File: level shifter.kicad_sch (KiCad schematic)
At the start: 81 parts, among them U501 TL074, U801 TL074

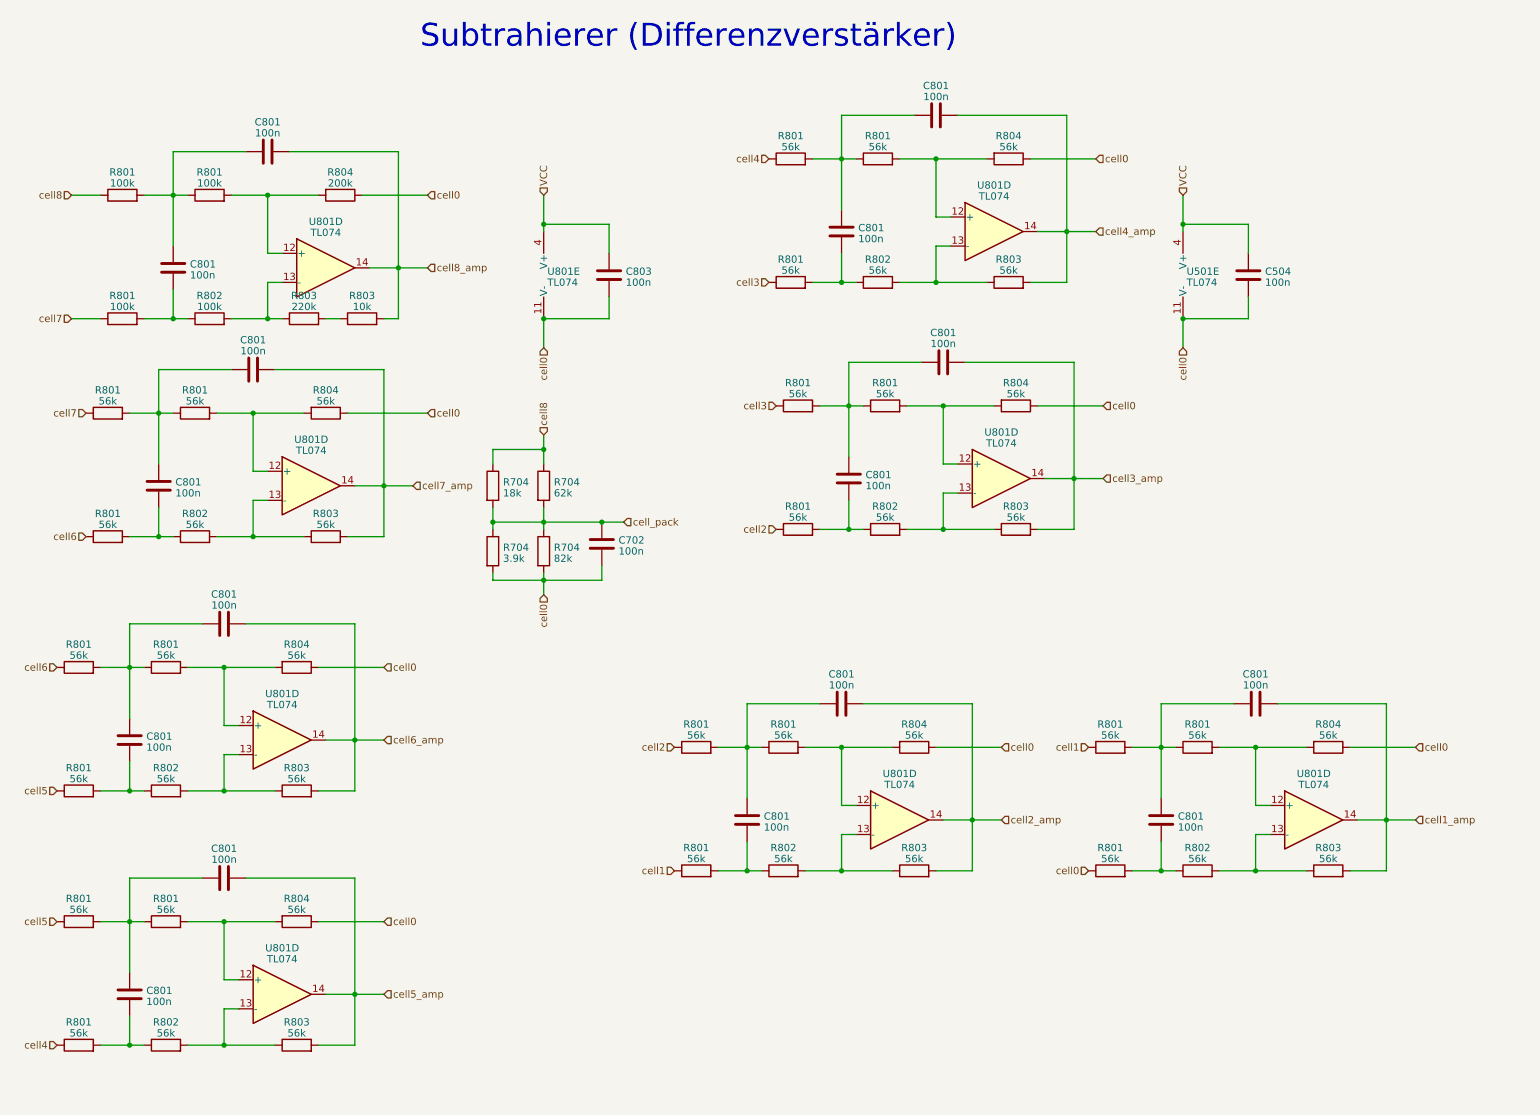
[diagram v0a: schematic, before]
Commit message: githubstart
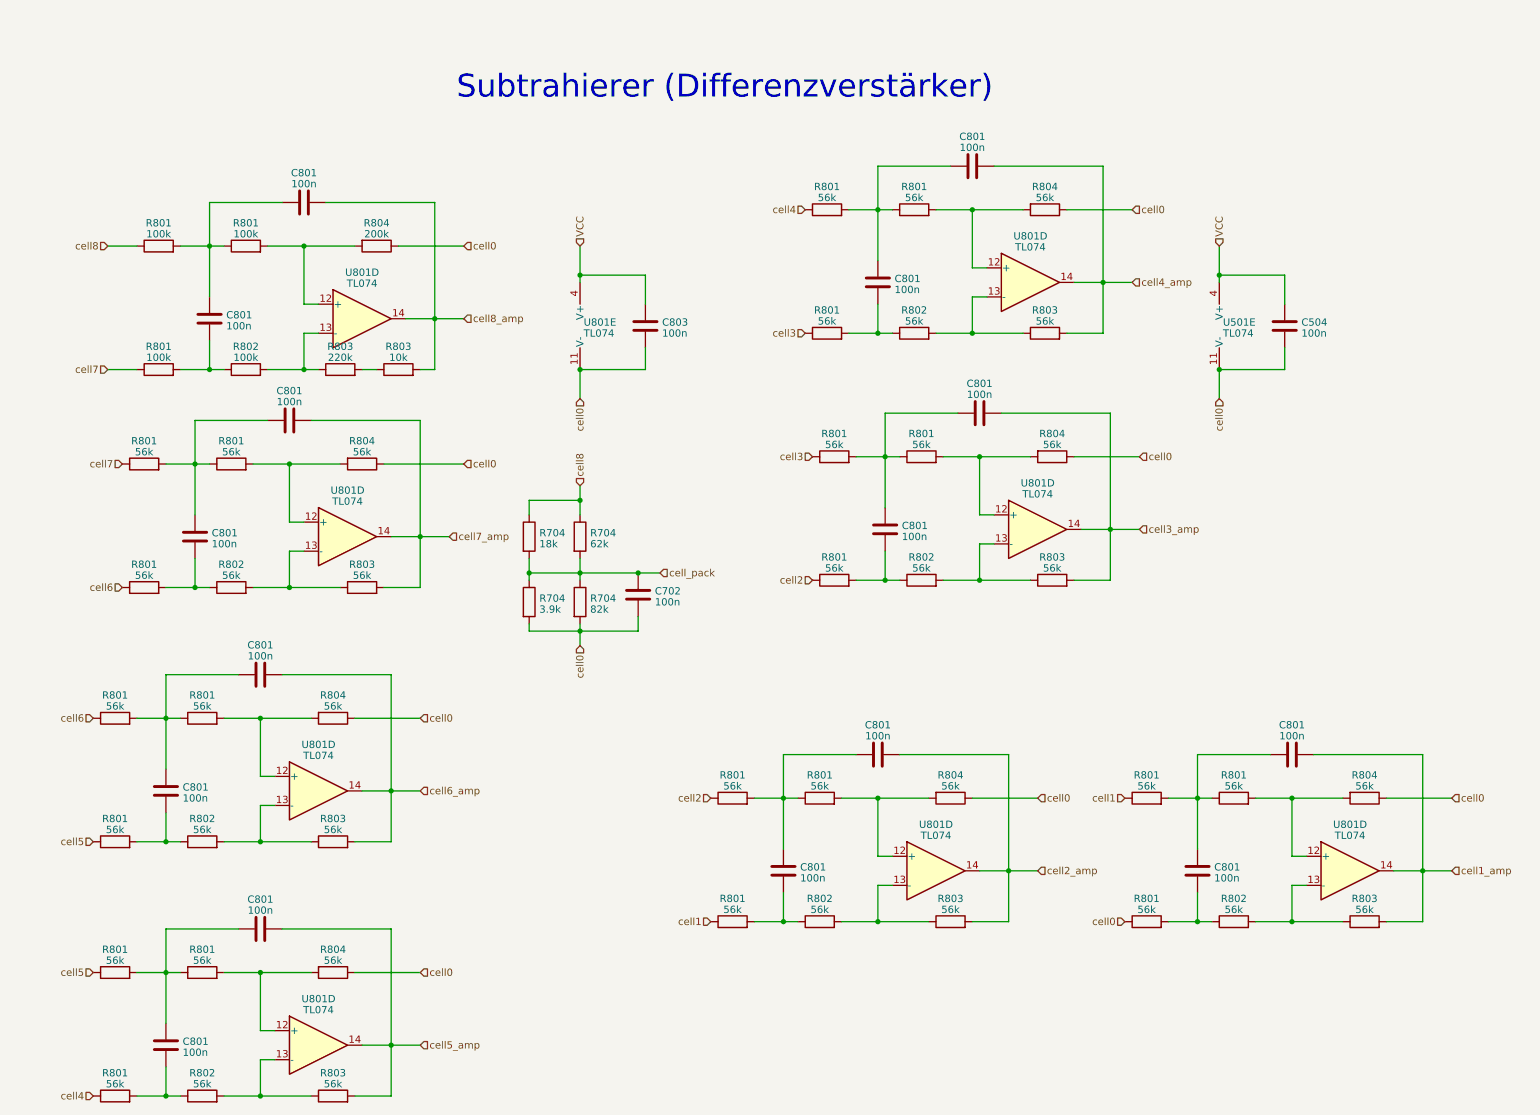
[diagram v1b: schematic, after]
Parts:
- removed C801 (x16): 100n, Capacitor_SMD:C_0603_1608Metric_Pad1.08x0.95mm_HandSolder, symbol Device:C
- removed R704: 3.9k, Resistor_SMD:R_0603_1608Metric_Pad0.98x0.95mm_HandSolder, symbol Device:R
- removed R704: 18k, Resistor_SMD:R_0603_1608Metric_Pad0.98x0.95mm_HandSolder, symbol Device:R
- removed R704: 82k, Resistor_SMD:R_0603_1608Metric_Pad0.98x0.95mm_HandSolder, symbol Device:R
- removed R704: 62k, Resistor_SMD:R_0603_1608Metric_Pad0.98x0.95mm_HandSolder, symbol Device:R
- removed R801 (x21), R802 (x7), R803 (x7), R804 (x7): 56k, Resistor_SMD:R_0603_1608Metric_Pad0.98x0.95mm_HandSolder, symbol Device:R
- removed R801 (x3), R802: 100k, Resistor_SMD:R_0603_1608Metric_Pad0.98x0.95mm_HandSolder, symbol Device:R
- removed R803: 220k, Resistor_SMD:R_0603_1608Metric_Pad0.98x0.95mm_HandSolder, symbol Device:R
- removed R803: 10k, Resistor_SMD:R_0603_1608Metric_Pad0.98x0.95mm_HandSolder, symbol Device:R
- removed R804: 200k, Resistor_SMD:R_0603_1608Metric_Pad0.98x0.95mm_HandSolder, symbol Device:R
- removed unit 4 of U801 (x8)
- added C801 (x16): 100n, Capacitor_SMD:C_0603_1608Metric_Pad1.08x0.95mm_HandSolder, symbol Device:C
- added R704: 82k, Resistor_SMD:R_0603_1608Metric_Pad0.98x0.95mm_HandSolder, symbol Device:R
- added R704: 62k, Resistor_SMD:R_0603_1608Metric_Pad0.98x0.95mm_HandSolder, symbol Device:R
- added R704: 18k, Resistor_SMD:R_0603_1608Metric_Pad0.98x0.95mm_HandSolder, symbol Device:R
- added R704: 3.9k, Resistor_SMD:R_0603_1608Metric_Pad0.98x0.95mm_HandSolder, symbol Device:R
- added R801 (x21), R802 (x7), R803 (x7), R804 (x7): 56k, Resistor_SMD:R_0603_1608Metric_Pad0.98x0.95mm_HandSolder, symbol Device:R
- added R801 (x3), R802: 100k, Resistor_SMD:R_0603_1608Metric_Pad0.98x0.95mm_HandSolder, symbol Device:R
- added R803: 10k, Resistor_SMD:R_0603_1608Metric_Pad0.98x0.95mm_HandSolder, symbol Device:R
- added R803: 220k, Resistor_SMD:R_0603_1608Metric_Pad0.98x0.95mm_HandSolder, symbol Device:R
- added R804: 200k, Resistor_SMD:R_0603_1608Metric_Pad0.98x0.95mm_HandSolder, symbol Device:R
- added unit 4 of U801 (x8)
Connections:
- net cell0: now also R704.2, R704.2, R801.1, R804.1, R804.1, R804.1, R804.1, R804.1, R804.1, R804.1, R804.1
- net cell1: now also R801.1, R801.1
- net cell1_amp: now also C801.1, R803.2, U801.14
- net cell2: now also R801.1, R801.1
- net cell2_amp: now also C801.1, R803.2, U801.14
- net cell3: now also R801.1, R801.1
- net cell3_amp: now also C801.1, R803.2, U801.14
- net cell4: now also R801.1, R801.1
- net cell4_amp: now also C801.1, R803.2, U801.14
- net cell5: now also R801.1, R801.1
- net cell5_amp: now also C801.1, R803.2, U801.14
- net cell6: now also R801.1, R801.1
- net cell6_amp: now also C801.1, R803.2, U801.14
- net cell7: now also R801.1, R801.1
- net cell7_amp: now also C801.1, R803.2, U801.14
- net cell8: now also R704.1, R704.1, R801.1
- net cell8_amp: now also C801.1, R803.2, U801.14
- net cell_pack: now also R704.1, R704.1, R704.2, R704.2
- new net: R801.2, R804.2, U801.12 (+) (x8)
- new net: R802.2, R803.1, U801.13 (-) (x8)
- new net: C801.1, R801.2, R802.1 (x8)
- new net: C801.2, C801.2, R801.1, R801.2 (x8)
- new net: R803.1, R803.2
